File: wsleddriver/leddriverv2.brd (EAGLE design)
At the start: 100 x 38.1 mm, 49 parts, among them IC1 WS2811-SOP8, IC2 WS2811-SOP8, IC3 WS2811-SOP8

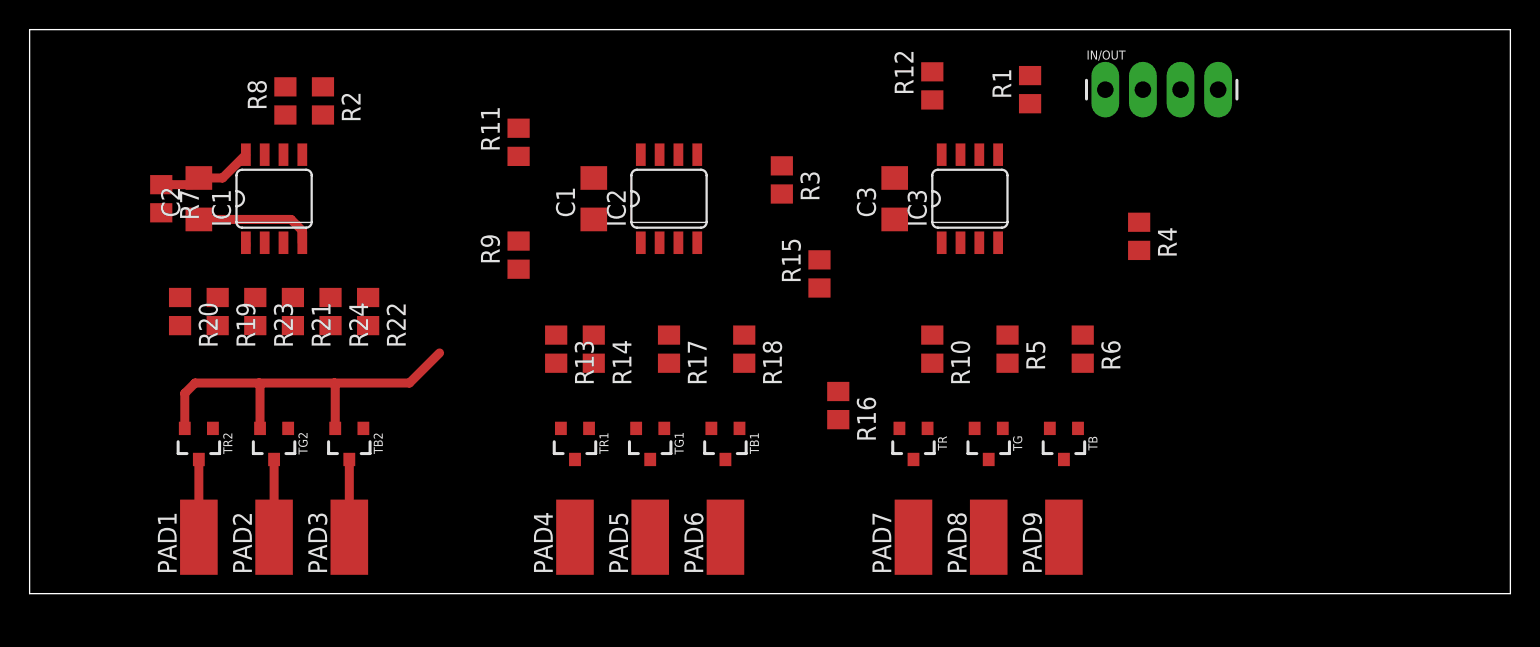
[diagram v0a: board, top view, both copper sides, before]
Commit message: c
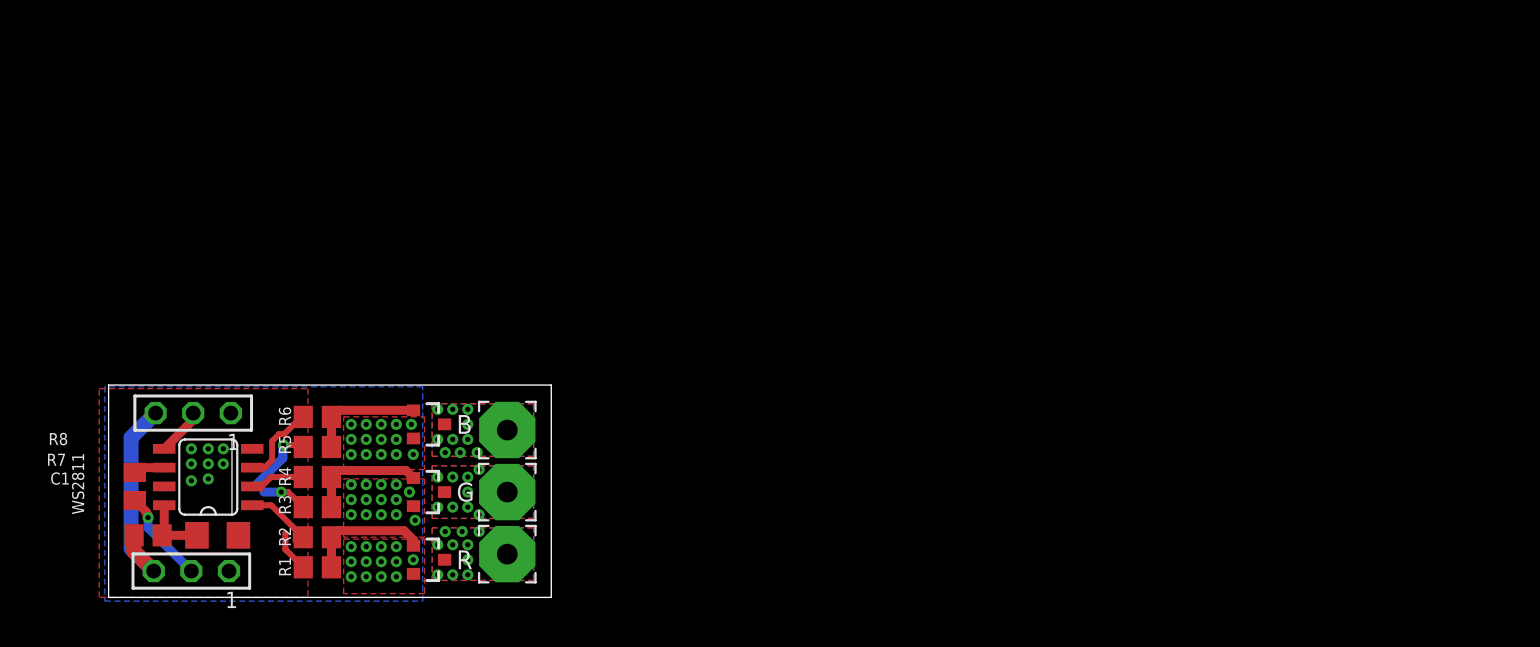
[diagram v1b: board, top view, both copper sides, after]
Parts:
- removed C2, C3: 0.1uF, rcl:C1206
- removed IC2, IC3: WS2811-SOP8, adafruit_wsled:SO08-SKINNYPADS
- removed IN/OUT: (no value), SparkFun-Connectors:1X04_LONGPADS
- removed PAD4, PAD5, PAD6, PAD7, PAD8, PAD9: (no value), wirepad:SMD2,54-5,08
- removed R10, R14, R17, R18, R20, R23, R24: 100, rcl:R0805
- removed R11, R12: 2.7k, rcl:R0805
- removed R13, R15, R16, R19, R21, R22, R9: 10k, rcl:R0805
- removed TB1, TB2, TG1, TG2, TR1, TR2: 5.8A/30V/35mΩ, SparkFun-DiscreteSemi:SOT23-3
- added X3, X4: TSW-103-07-G-S, con-samtec:TSW-103-XX-G-S
- PAD1, PAD2, PAD3: device wirepad:SMD2,54-5,08 -> wirepad:3,81/1,4
- R1: value 33 -> 10k
- R2: value 33 -> 100
- R4: value 10k -> 100
- R5: value 100 -> 10k
- moved R1 57.9 mm to (19.4, 1.78), turned to 0 degrees
- moved R4 57.8 mm to (19.4, 7.87), turned to 0 degrees
- moved R6 51.9 mm to (19.4, 11.9), turned to 0 degrees
- moved R5 47.1 mm to (19.4, 9.91), turned to 0 degrees
- moved TB 42.9 mm to (26.9, 11.4), turned to 270 degrees
- moved R3 38.4 mm to (19.4, 5.84), turned to 0 degrees
- moved TG 38.0 mm to (26.9, 6.86), turned to 270 degrees
- moved C1 34.1 mm to (12.7, 3.94), turned to 180 degrees
- moved TR 33.7 mm to (26.9, 2.29), turned to 270 degrees
- moved R2 29.5 mm to (19.4, 3.81), turned to 0 degrees
- moved R8 27.9 mm to (7.11, 7.24), turned to 270 degrees
- moved R7 22.8 mm to (8.00, 3.94), turned to 180 degrees
- moved PAD1 20.9 mm to (32.3, 2.67)
- moved IC1 19.3 mm to (12.1, 7.87), turned to 90 degrees
- moved PAD2 16.0 mm to (32.3, 6.86)
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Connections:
- removed net B2: IC2.3, R18.1
- removed net B3: IC3.3, R6.1
- removed net G2: IC2.2, R17.1
- removed net G3: IC3.2, R5.1
- removed net N$10: R21.2, R23.2, TG2.1
- removed net N$11: IC2.5, R1.2
- removed net N$12: R22.2, R24.2, TB2.1
- removed net N$13: IC3.6, R1.1
- removed net N$14: IC2.6, R2.1
- removed net N$5: IC1.5, R2.2
- removed net N$6: R13.2, R14.2, TR1.1
- removed net N$7: R15.2, R17.2, TG1.1
- removed net N$8: R16.2, R18.2, TB1.1
- removed net N$9: R19.2, R20.2, TR2.1
- removed net NEG_B2: TB1.3
- removed net NEG_B3: TB.3
- removed net NEG_G2: TG1.3
- removed net NEG_G3: TG.3
- removed net NEG_R2: TR1.3
- removed net NEG_R3: TR.3
- removed net R2: IC2.1, R14.1
- removed net R3: IC3.1, R10.1
- net +12V: now also R1.1, R5.1, X3.3, X4.3; no longer IN/OUT.4, R11.2, R12.2, R13.1, R15.1, R16.1, R19.1, R21.1, R22.1, R4.1, R9.1
- net B: now also R6.1; no longer R24.1
- net DIN_IN: now also X3.2; no longer IN/OUT.3
- net DOUT_OUT: now also IC1.5, X4.2; no longer IC3.5, IN/OUT.2
- net G: now also R4.1; no longer R23.1
- net GND: now also X3.1, X4.1; no longer C2.1, C3.1, IC2.4, IC3.4, IN/OUT.1, TB1.2, TB2.2, TG1.2, TG2.2, TR1.2, TR2.2
- net N$2: now also R4.2; no longer R5.2
- net N$3: now also R5.2; no longer R4.2
- net N$4: now also R1.2, R2.2; no longer R10.2, R9.2
- net NEG_B: now also TB.3; no longer TB2.3
- net NEG_G: now also TG.3; no longer TG2.3
- net NEG_R: now also TR.3; no longer TR2.3
- net R: now also R2.1; no longer R20.1
- net VDD: no longer C2.2, C3.2, IC2.8, IC3.8, R11.1, R12.1
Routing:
- net GND: track 35.0 -> 0.00 mm, vias 0 -> 49
- net +12V: track 0.00 -> 25.7 mm, vias 0 -> 2
- net N$4: track 0.00 -> 8.40 mm
- net N$2: track 0.00 -> 7.97 mm
- net N$3: track 0.00 -> 7.76 mm
- net DIN_IN: track 0.00 -> 6.34 mm, vias 0 -> 1
- net B: track 0.00 -> 5.62 mm
- net NEG_R: track 5.25 -> 0.00 mm, vias 0 -> 10
- net NEG_G: track 5.25 -> 0.00 mm, vias 0 -> 9
- net NEG_B: track 5.25 -> 0.00 mm, vias 0 -> 10
- net R: track 0.20 -> 5.37 mm
- net G: track 0.00 -> 4.10 mm
- net DOUT_OUT: track 0.00 -> 3.22 mm
- net N$1: track 0.00 -> 2.21 mm
- net VDD: track 6.55 -> 4.43 mm
- added copper zone on layer 1, net GND
- added copper zone on layer 16, net GND
- added copper zone on layer 1, net NEG_B
- added copper zone on layer 16, net NEG_B
- added copper zone on layer 1, net NEG_G
- added copper zone on layer 16, net NEG_G
- added copper zone on layer 1, net NEG_R
- added copper zone on layer 16, net NEG_R
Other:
- board size 100 x 38.1 mm -> 29.9 x 14.3 mm
- board text added: "B"
- board text added: "C1"
- board text added: "G"
- board text added: "R"
- board text added: "R1"
- board text added: "R2"
- board text added: "R3"
- board text added: "R4"
- board text added: "R5"
- board text added: "R6"
- board text added: "R7"
- board text added: "R8"
- board text added: "WS2811"
